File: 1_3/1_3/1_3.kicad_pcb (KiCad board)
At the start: 2 copper layers, 137.5 x 93.4 mm, 52 parts, among them SW1 SW_SPST, SW10 SW_SPST, SW11 SW_SPST, SW12 SW_SPST, SW13 SW_SPST, SW14 SW_SPST, SW15 SW_SPST, SW16 SW_SPST, SW17 SW_SPST, SW18 SW_SPST, SW19 SW_SPST, SW2 SW_SPST, SW20 SW_SPST, SW21 SW_SPST, SW3 SW_SPST, SW4 SW_SPST, SW5 SW_SPST, SW6 SW_SPST, SW7 SW_SPST, SW8 SW_SPST, SW9 SW_SPST, U1 XIAO_nRF52840

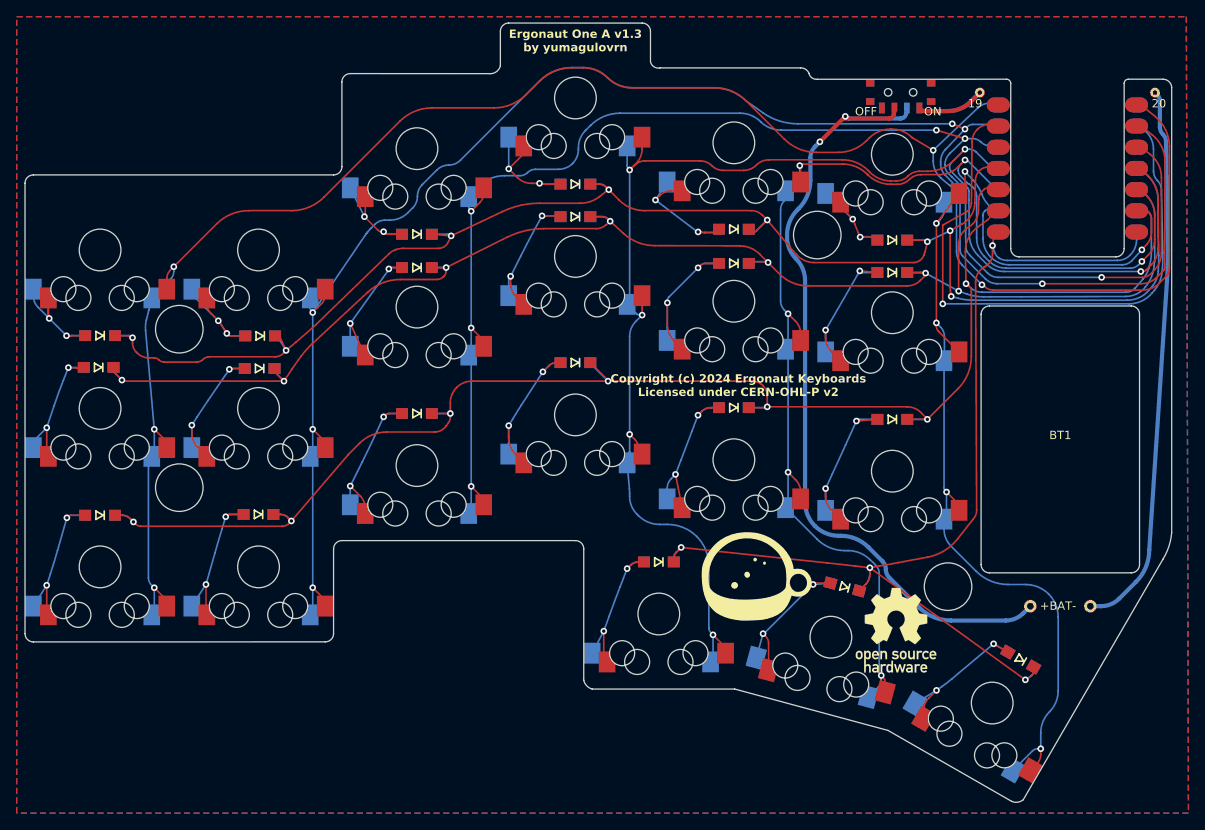
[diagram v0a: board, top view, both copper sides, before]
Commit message: 1_3
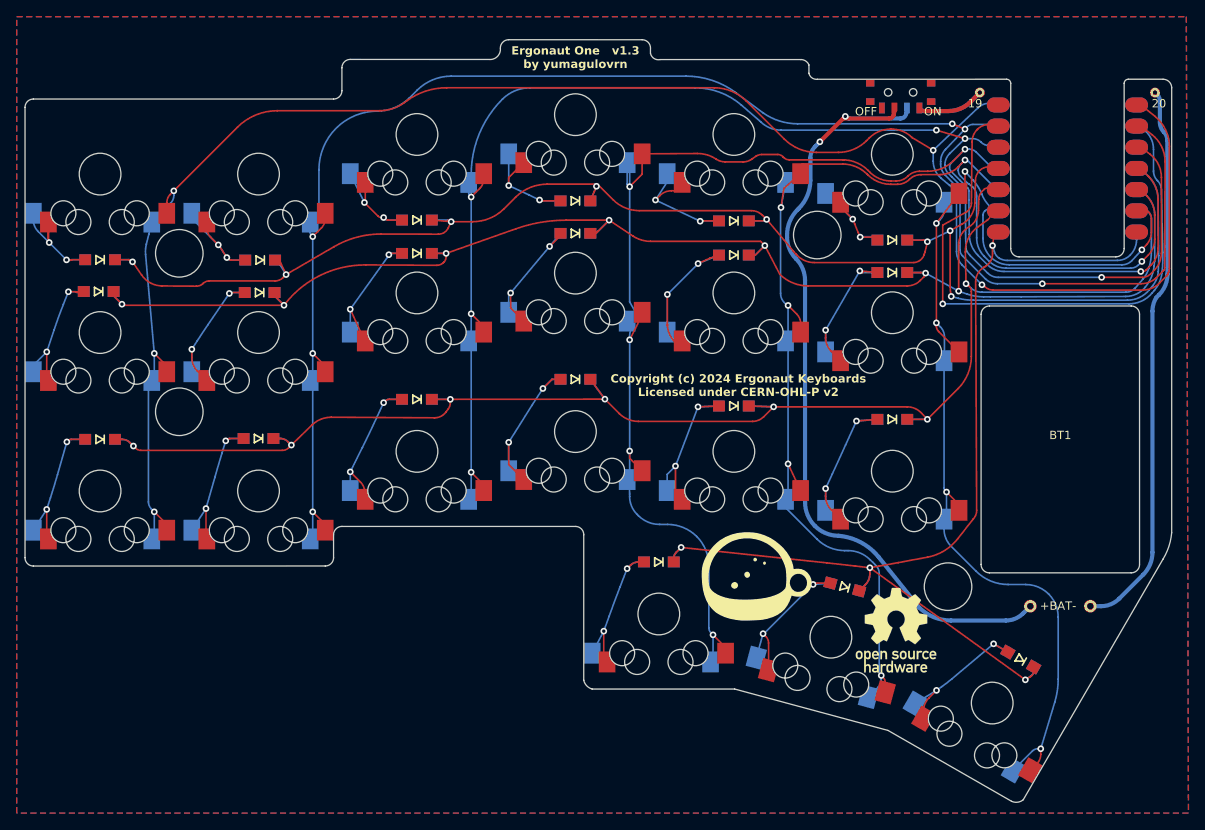
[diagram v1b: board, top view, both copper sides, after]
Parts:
- moved D13 9.10 mm to (84.5, 98.8)
- moved D2 9.10 mm to (103.7, 77.3)
- moved D7 9.10 mm to (84.3, 81.1)
- moved D1 9.10 mm to (84.5, 77.3)
- moved D14 9.10 mm to (103.5, 98.7)
- moved D8 9.10 mm to (103.6, 81.2)
- moved H1 9.10 mm to (94.0, 76.5)
- moved H2 9.10 mm to (94.0, 95.5)
- moved SW1 9.10 mm to (84.5, 67.0)
- moved SW13 9.10 mm to (84.5, 105.0)
- moved SW14 9.10 mm to (103.5, 105.0)
- moved SW2 9.10 mm to (103.5, 67.0)
- moved SW7 9.10 mm to (84.5, 86.0)
- moved SW8 9.10 mm to (103.5, 86.0)
- moved D10 2.00 mm to (141.5, 74.1)
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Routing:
- net C2: track 166.2 -> 172.1 mm
- net R2: track 196.2 -> 190.7 mm
- net R0: track 198.9 -> 193.6 mm
- net C0: track 225.4 -> 220.5 mm
- net C1: track 202.6 -> 199.9 mm
- net Net-(D16-A): track 18.9 -> 21.4 mm
- net R1: track 185.0 -> 183.0 mm
- net Net-(D11-A): track 19.5 -> 21.3 mm
- net Net-(D17-A): track 20.6 -> 19.2 mm
- net Net-(D10-A): track 18.9 -> 17.6 mm
- net Net-(D5-A): track 17.5 -> 16.6 mm
- net Net-(D18-A): track 21.7 -> 20.9 mm
- net C3: track 173.7 -> 174.5 mm
- net Net-(D4-A): track 15.7 -> 16.5 mm
- net Net-(BT1--): track 66.1 -> 66.7 mm
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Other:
- board size 137.5 x 93.4 mm -> 137.5 x 91.4 mm
- board text added: "Ergonaut One v1.3 by yumagulovrn"
- board text removed: "Ergonaut One A v1.3 by yumagulovrn"
